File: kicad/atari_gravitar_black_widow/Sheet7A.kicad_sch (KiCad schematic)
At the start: 28 parts

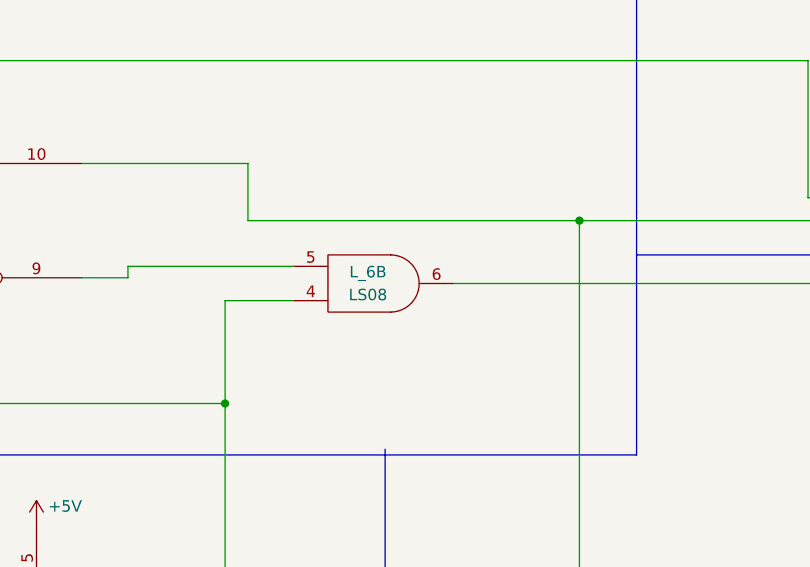
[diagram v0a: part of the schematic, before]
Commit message: first traces.
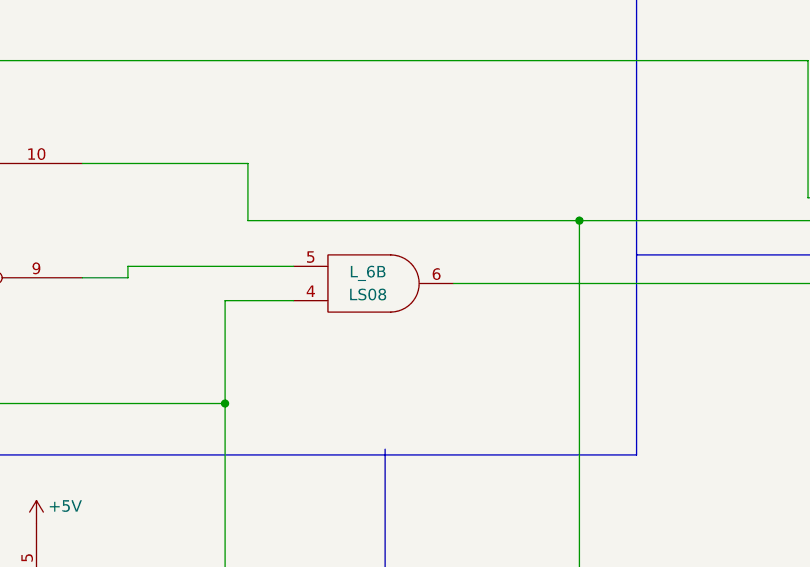
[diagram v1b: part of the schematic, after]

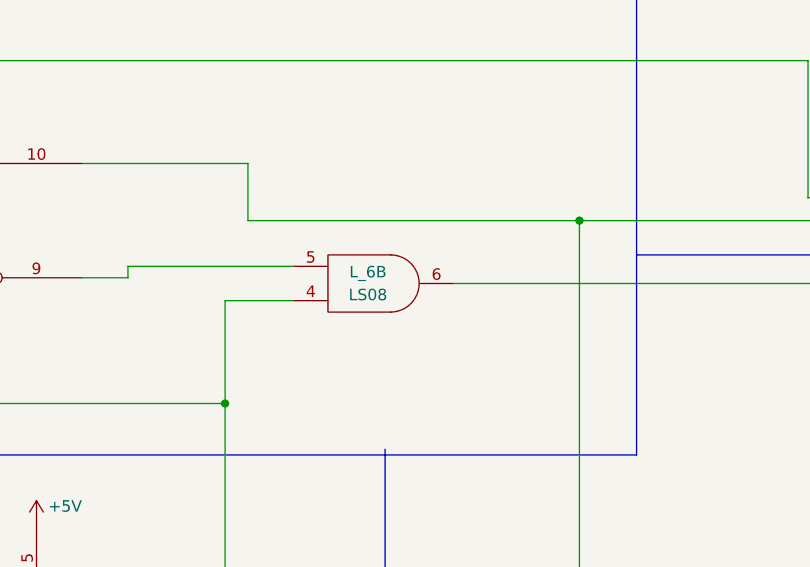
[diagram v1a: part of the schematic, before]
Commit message: test traces
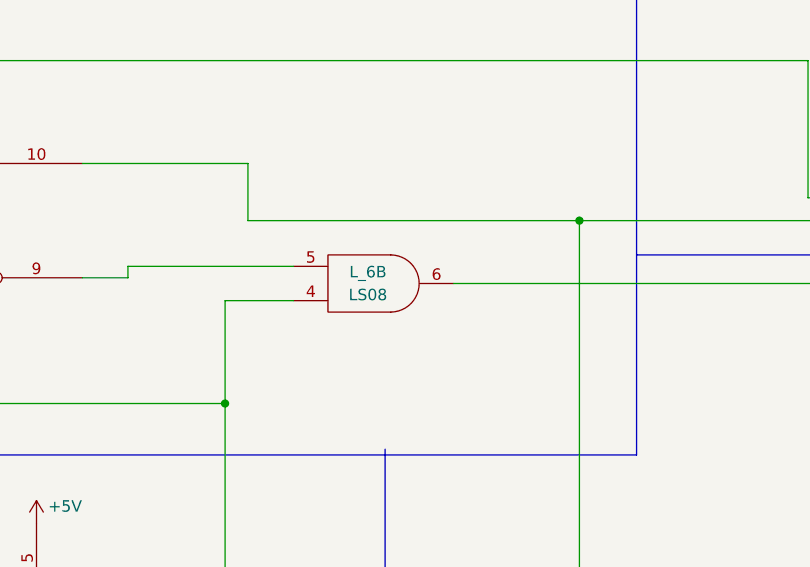
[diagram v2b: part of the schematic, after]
